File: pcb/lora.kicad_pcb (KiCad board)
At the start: 4 copper layers, 80.5 x 45 mm, 51 parts, among them J11 Conn_Coaxial, J2 Humidity, J3 Temp, J5 Temp, J6 VDD, J7 GPS, J8 SIM800, J9 I2C, Q1 AO3401A, Q2 AO3401A, Q3 AO3401A, Q5 AO3401A, SW1 RESET, SW2 PJ, U2 ESP32-WROOM-32D, U3 2460, U4 RFM95W-868S2, Y1 Crystal

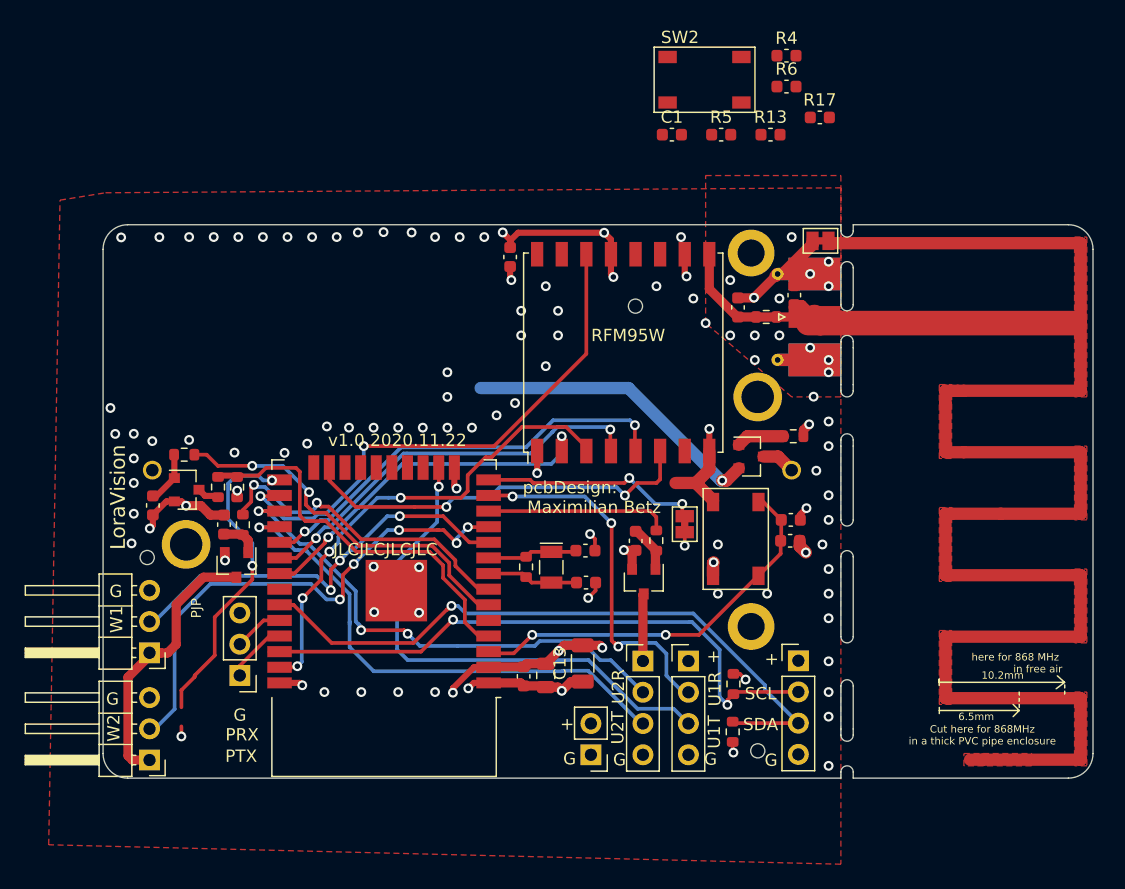
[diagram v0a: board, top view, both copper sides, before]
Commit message: figured all GPIOs out
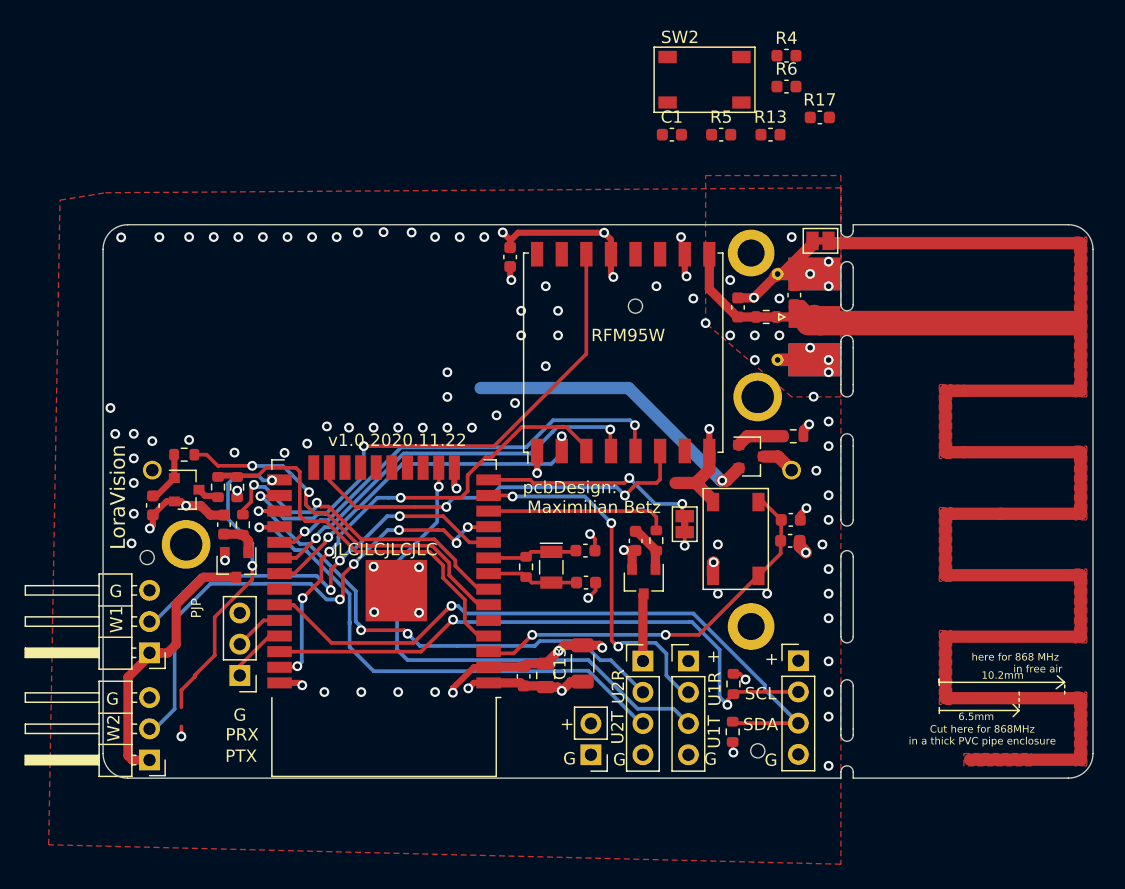
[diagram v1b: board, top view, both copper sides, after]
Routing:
- added copper zone on In1.Cu, net GND
- added copper zone on In2.Cu, net VBATT
- removed copper zone on In1.Cu_GND, net GND
- removed copper zone on In2.Cu_VDD, net VBATT
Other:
- net class Default removed
